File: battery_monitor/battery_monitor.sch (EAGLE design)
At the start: 36 parts, among them CON1 SM04B-GHS-TB, CON2 SM04B-GHS-TB, J1 2PIN_HDR, U1 STM32F303CB

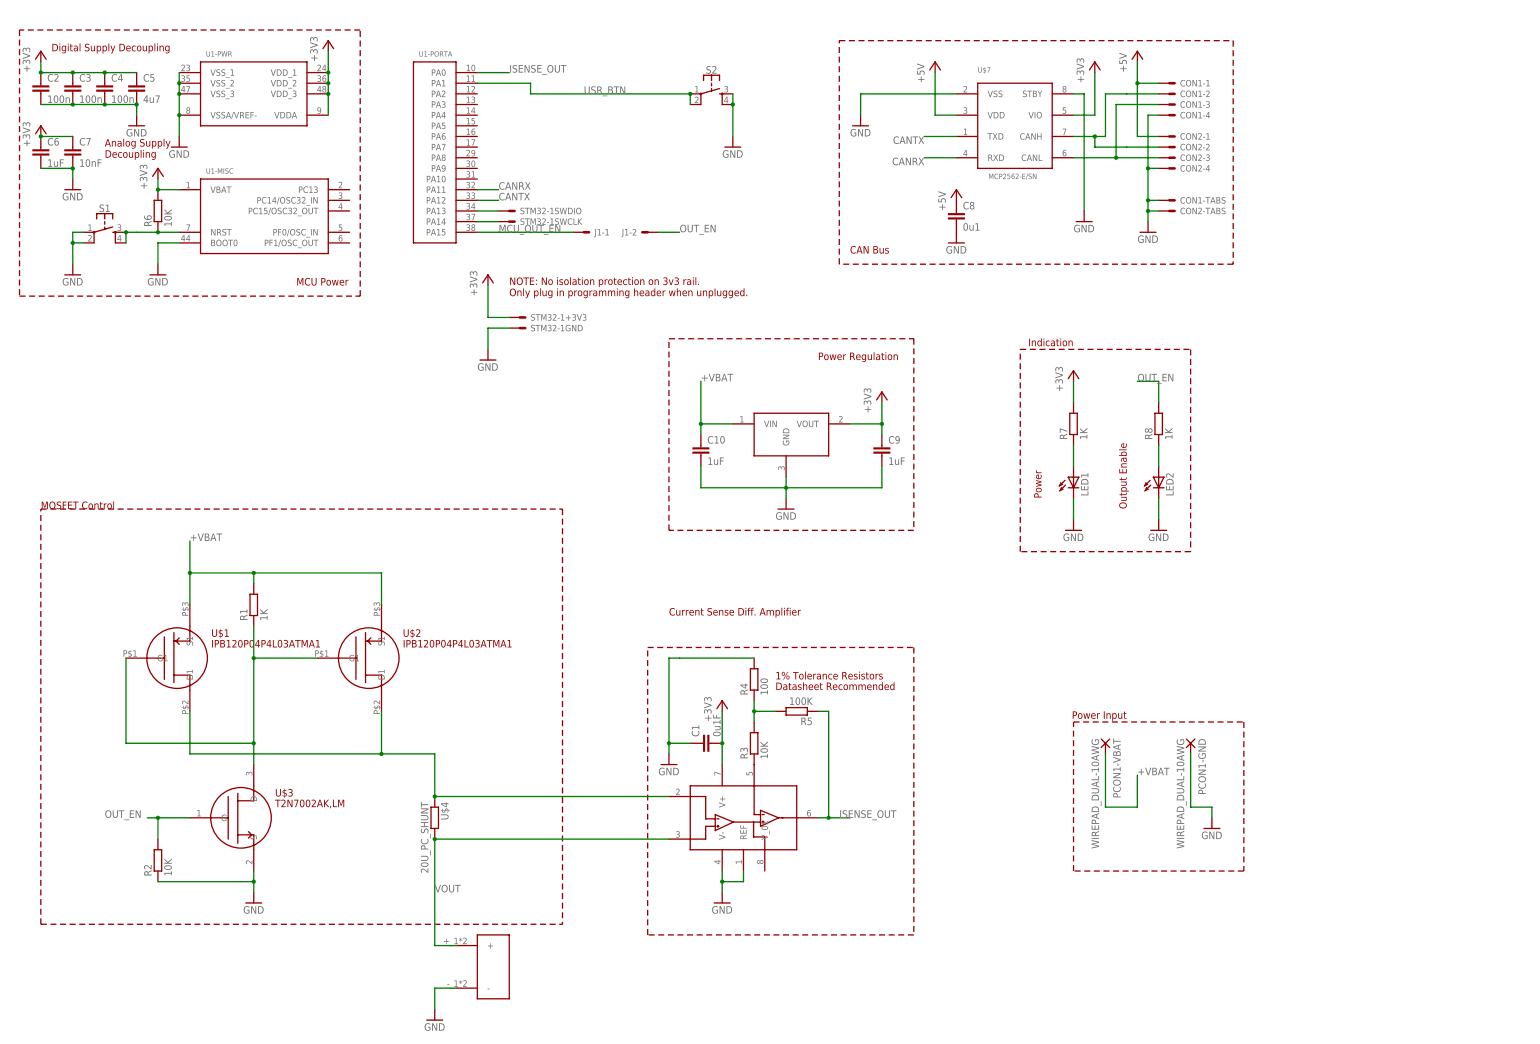
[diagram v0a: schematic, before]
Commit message: Updated battery monitor design.
- Added cortex debug header.
- Added voltage divider to read voltage from batteries.
- Added 8MHz crystal oscillator
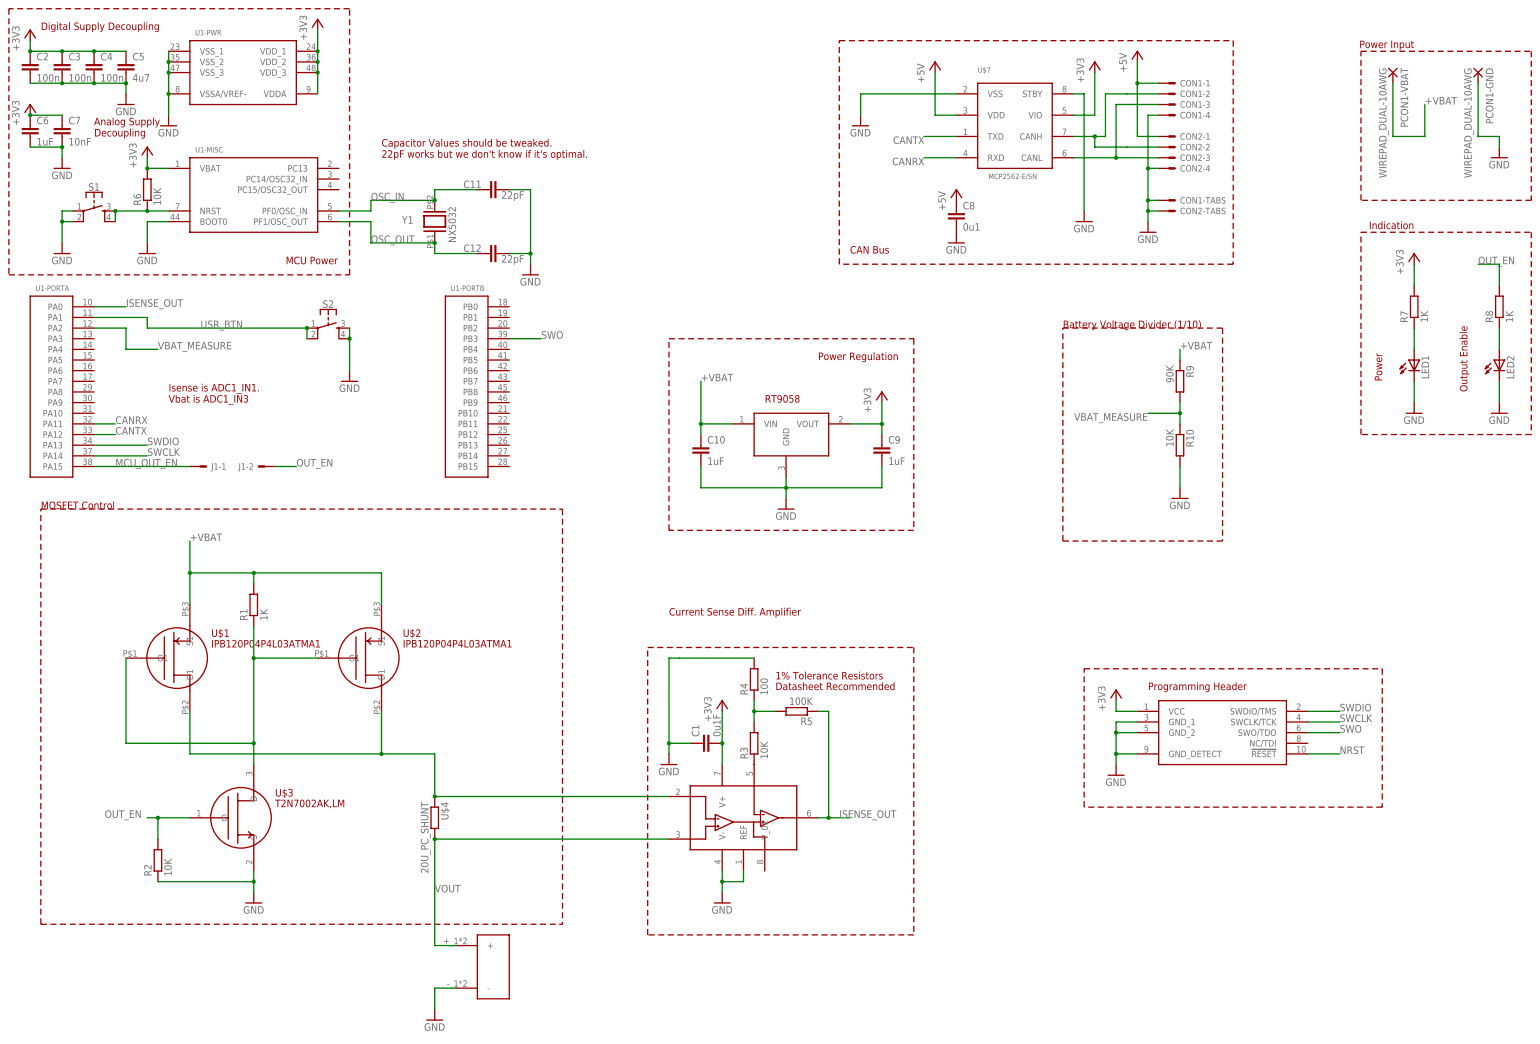
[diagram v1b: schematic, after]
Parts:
- removed STM32-1: STM32_SWD-HDR, SPEAR-battery-monitor:STM32_SWD-HDR
- added C11, C12: 22pF, resistor:C-EUC0805
- added JP1: CORTEX-M-DBG, SPEAR-general:CORTEX-M-DBG
- added R10: 10K, resistor:R-EU_R0805
- added R9: 90K, resistor:R-EU_R0805
- added Y1: NX5032, SPEAR-general:NX5032
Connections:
- removed net N$5: STM32-1SWDIO.S, U1-PORTA.PA13
- removed net N$6: STM32-1SWCLK.S, U1-PORTA.PA14
- new net OSC_IN: C11.1, U1-MISC.PF0/OSC_IN, Y1.2
- new net OSC_OUT: C12.1, U1-MISC.PF1/OSC_OUT, Y1.1
- new net SWCLK: JP1.SWCLK/TCK, U1-PORTA.PA14
- new net SWDIO: JP1.SWDIO/TMS, U1-PORTA.PA13
- new net SWO: JP1.SWO/TDO, U1-PORTB.PB3
- new net VBAT_MEASURE: R10.1, R9.2, U1-PORTA.PA2
- net +3V3: now also JP1.VCC; no longer STM32-1+3V3.S
- net +VBAT: now also R9.1
- net GND: now also C11.2, C12.2, JP1.GND_1, JP1.GND_2, JP1.GND_DETECT, R10.2; no longer STM32-1GND.S
- net NRST: now also JP1.!RESET
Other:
- note added: "Battery Voltage Divider (1/10)"
- note added: "Capacitor Values should be tweaked. 22pF works but we don't know if it's optimal."
- note added: "Isense is ADC1_IN1. Vbat is ADC1_IN3"
- note added: "Programming Header"
- note added: "RT9058"
- note removed: "NOTE: No isolation protection on 3v3 rail. Only plug in programming header when unplugged."
- moved on the sheet: C2, C3, C4, C5, C6, C7, J1-1, J1-2, LED1, LED2, PCON1-GND, PCON1-VBAT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
